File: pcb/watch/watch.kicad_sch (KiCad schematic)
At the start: 106 parts

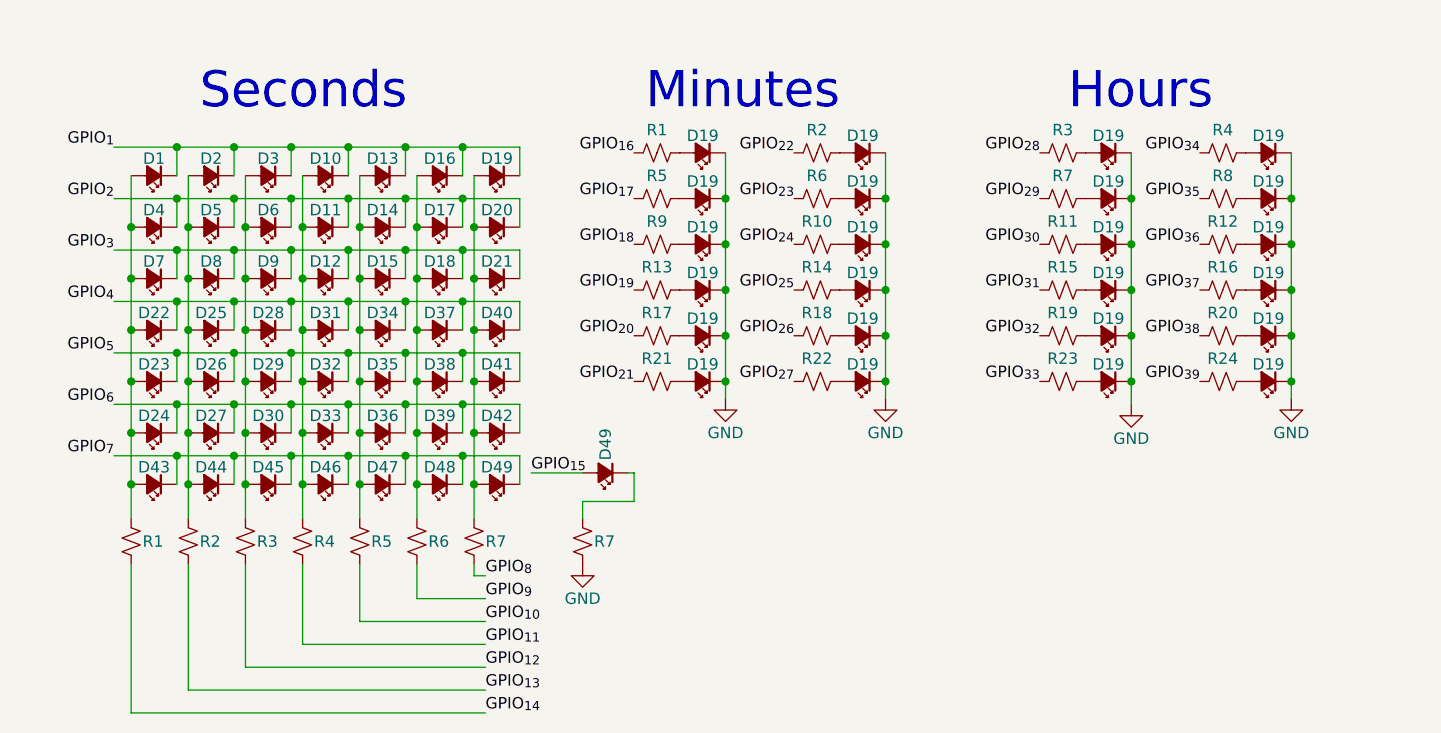
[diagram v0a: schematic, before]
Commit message: fuck fuck fuck I made it too small
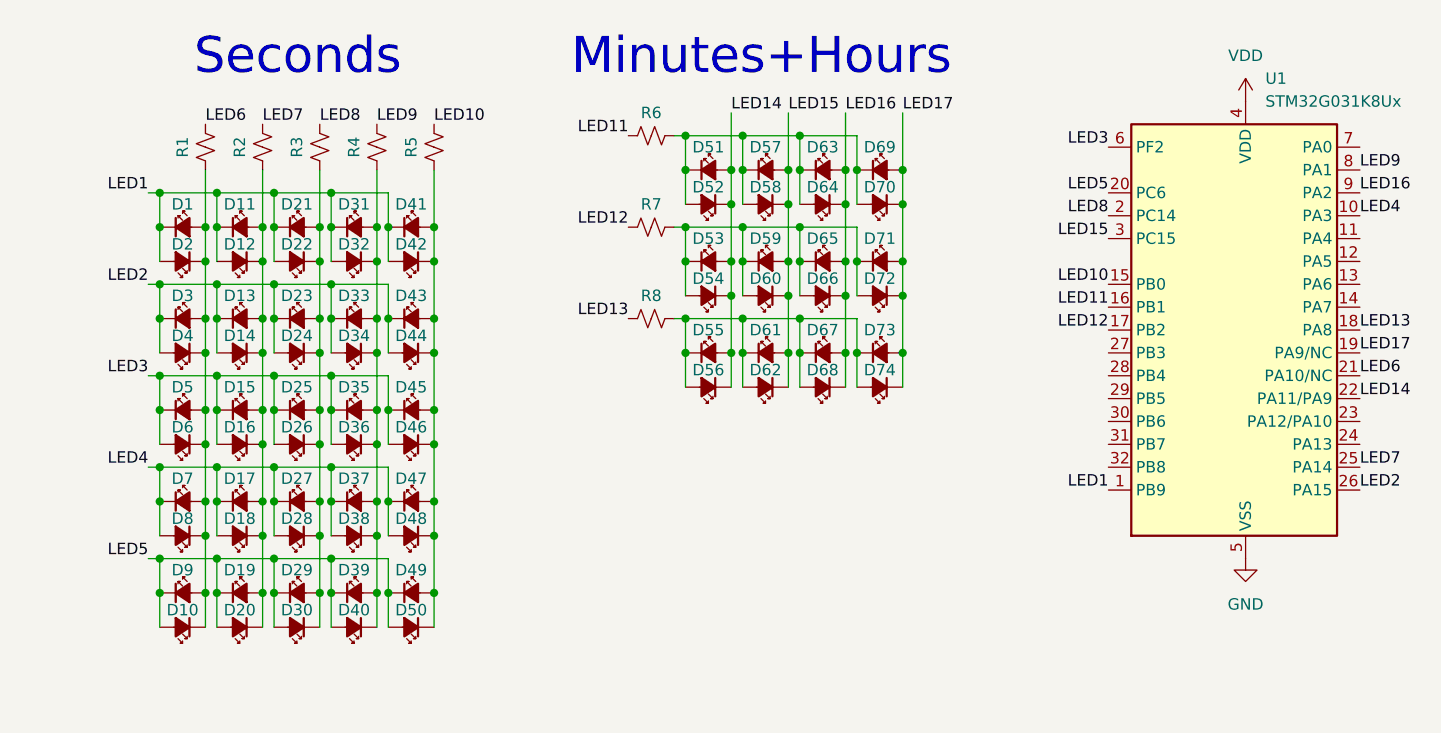
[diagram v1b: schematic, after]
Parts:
- removed D19 (x25), D49 (x2): LED_Small_Filled, LED_SMD:LED_0402_1005Metric, symbol Device:LED_Small_Filled
- removed R1 (x2), R10, R11, R12, R13, R14, R15, R16, R17, R18, R19, R2 (x2), R20, R21, R22, R23, R24, R3 (x2), R4 (x2), R5 (x2), R6 (x2), R7 (x3), R9: R_Small_US, Resistor_SMD:R_0402_1005Metric, symbol Device:R_Small_US
- added D19, D49, D50, D51, D52, D53, D54, D55, D56, D57, D58, D59, D60, D61, D62, D63, D64, D65, D66, D67, D68, D69, D70, D71, D72, D73, D74: LED_Small_Filled, LED_SMD:LED_0402_1005Metric, symbol Device:LED_Small_Filled
- added R1, R2, R3, R4, R5, R6, R7: R_Small_US, Resistor_SMD:R_0402_1005Metric, symbol Device:R_Small_US
- added U1: STM32G031K8Ux, Package_DFN_QFN:UFQFPN-32-1EP_5x5mm_P0.5mm_EP3.5x3.5mm, symbol MCU_ST_STM32G0:STM32G031K8Ux
- D1, D11, D21, D31, D41: footprint LED_SMD:LED_0402_1005Metric -> footprints:LED_0402_1005Metric
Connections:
- net GND: now also U1.33 (VSS), U1.5 (VSS)
- net at R8.2: now also D55.1 (K), D56.2 (A), D61.1 (K), D62.2 (A), D67.1 (K), D68.2 (A), D73.1 (K), D74.2 (A)
- removed net GPIO_{1}: D1.1 (K), D10.1 (K), D13.1 (K), D16.1 (K), D2.1 (K), D3.1 (K)
- removed net GPIO_{2}: D11.1 (K), D14.1 (K), D17.1 (K), D20.1 (K), D4.1 (K), D5.1 (K), D6.1 (K)
- net GPIO_{35} renamed LED13
- net LED13: now also U1.18 (PA8)
- removed net GPIO_{3}: D12.1 (K), D15.1 (K), D18.1 (K), D21.1 (K), D7.1 (K), D8.1 (K), D9.1 (K)
- removed net GPIO_{4}: D22.1 (K), D25.1 (K), D28.1 (K), D31.1 (K), D34.1 (K), D37.1 (K), D40.1 (K)
- removed net GPIO_{5}: D23.1 (K), D26.1 (K), D29.1 (K), D32.1 (K), D35.1 (K), D38.1 (K), D41.1 (K)
- removed net GPIO_{6}: D24.1 (K), D27.1 (K), D30.1 (K), D33.1 (K), D36.1 (K), D39.1 (K), D42.1 (K)
- net GPIO_{7}: no longer names the net of D44.1 (K), D46.1 (K), D48.1 (K)
- net GPIO_{7}: now also D41.2 (A), D42.1 (K), D43.2 (A), D45.2 (A), D47.2 (A), D49.2 (A), D50.1 (K), R5.1; no longer D43.1 (K), D45.1 (K), D47.1 (K)
- new net: D53.1 (K), D54.2 (A), D59.1 (K), D60.2 (A), D65.1 (K), D66.2 (A), D71.1 (K), D72.2 (A), R7.2
- new net: D1.2 (A), D10.1 (K), D2.1 (K), D3.2 (A), D4.1 (K), D5.2 (A), D6.1 (K), D7.2 (A), D8.1 (K), D9.2 (A), R1.1
- new net: D11.2 (A), D12.1 (K), D13.2 (A), D14.1 (K), D15.2 (A), D16.1 (K), D17.2 (A), D18.1 (K), D19.2 (A), D20.1 (K), R2.1
- new net: D31.2 (A), D32.1 (K), D33.2 (A), D34.1 (K), D35.2 (A), D36.1 (K), D37.2 (A), D38.1 (K), D39.2 (A), D40.1 (K), R4.1
- new net: D51.1 (K), D52.2 (A), D57.1 (K), D58.2 (A), D63.1 (K), D64.2 (A), D69.1 (K), D70.2 (A), R6.2
- new net: D21.2 (A), D22.1 (K), D23.2 (A), D24.1 (K), D25.2 (A), D26.1 (K), D27.2 (A), D28.1 (K), D29.2 (A), D30.1 (K), R3.1
- new net LED1: D1.1 (K), D11.1 (K), D12.2 (A), D2.2 (A), D21.1 (K), D22.2 (A), D31.1 (K), D32.2 (A), D41.1 (K), D42.2 (A), U1.1 (PB9)
- new net LED10: R5.2, U1.15 (PB0)
- new net LED11: R6.1, U1.16 (PB1)
- new net LED12: R7.1, U1.17 (PB2)
- new net LED14: D51.2 (A), D52.1 (K), D53.2 (A), D54.1 (K), D55.2 (A), D56.1 (K), U1.22 (PA11/PA9)
- new net LED15: D57.2 (A), D58.1 (K), D59.2 (A), D60.1 (K), D61.2 (A), D62.1 (K), U1.3 (PC15)
- new net LED16: D63.2 (A), D64.1 (K), D65.2 (A), D66.1 (K), D67.2 (A), D68.1 (K), U1.9 (PA2)
- new net LED17: D69.2 (A), D70.1 (K), D71.2 (A), D72.1 (K), D73.2 (A), D74.1 (K), U1.19 (PA9/NC)
- new net LED2: D13.1 (K), D14.2 (A), D23.1 (K), D24.2 (A), D3.1 (K), D33.1 (K), D34.2 (A), D4.2 (A), D43.1 (K), D44.2 (A), U1.26 (PA15)
- new net LED3: D15.1 (K), D16.2 (A), D25.1 (K), D26.2 (A), D35.1 (K), D36.2 (A), D45.1 (K), D46.2 (A), D5.1 (K), D6.2 (A), U1.6 (PF2)
- new net LED4: D17.1 (K), D18.2 (A), D27.1 (K), D28.2 (A), D37.1 (K), D38.2 (A), D47.1 (K), D48.2 (A), D7.1 (K), D8.2 (A), U1.10 (PA3)
- new net LED5: D10.2 (A), D19.1 (K), D20.2 (A), D29.1 (K), D30.2 (A), D39.1 (K), D40.2 (A), D49.1 (K), D50.2 (A), D9.1 (K), U1.20 (PC6)
- new net LED6: R1.2, U1.21 (PA10/NC)
- new net LED7: R2.2, U1.25 (PA14)
- new net LED8: R3.2, U1.2 (PC14)
- new net LED9: R4.2, U1.8 (PA1)
- new net VDD: U1.4 (VDD)
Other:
- note added: "Minutes+Hours"
- note removed: "Hours"
- note removed: "Minutes"
